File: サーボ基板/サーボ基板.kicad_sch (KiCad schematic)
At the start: 22 parts, among them J1 Conn_01x02, J2 Conn_01x03, J3 Conn_01x03, J4 Conn_01x03, J5 Conn_01x03, J6 DATA_IN, U1 SeeeduinoXIAO RP2040

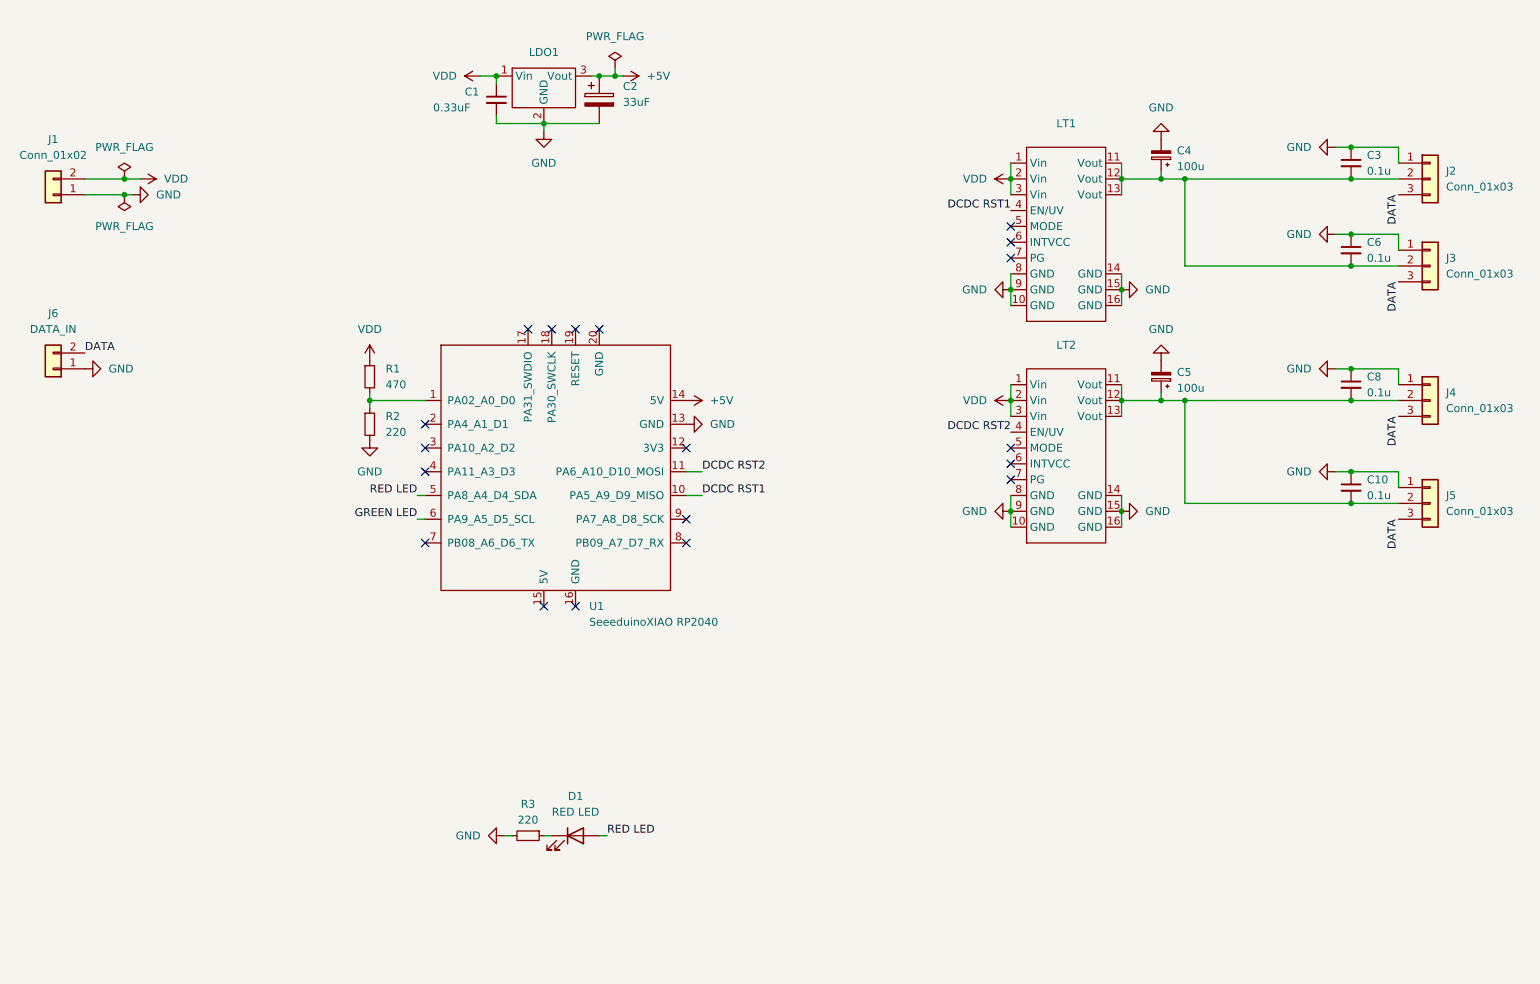
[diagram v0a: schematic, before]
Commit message: サーボ基板
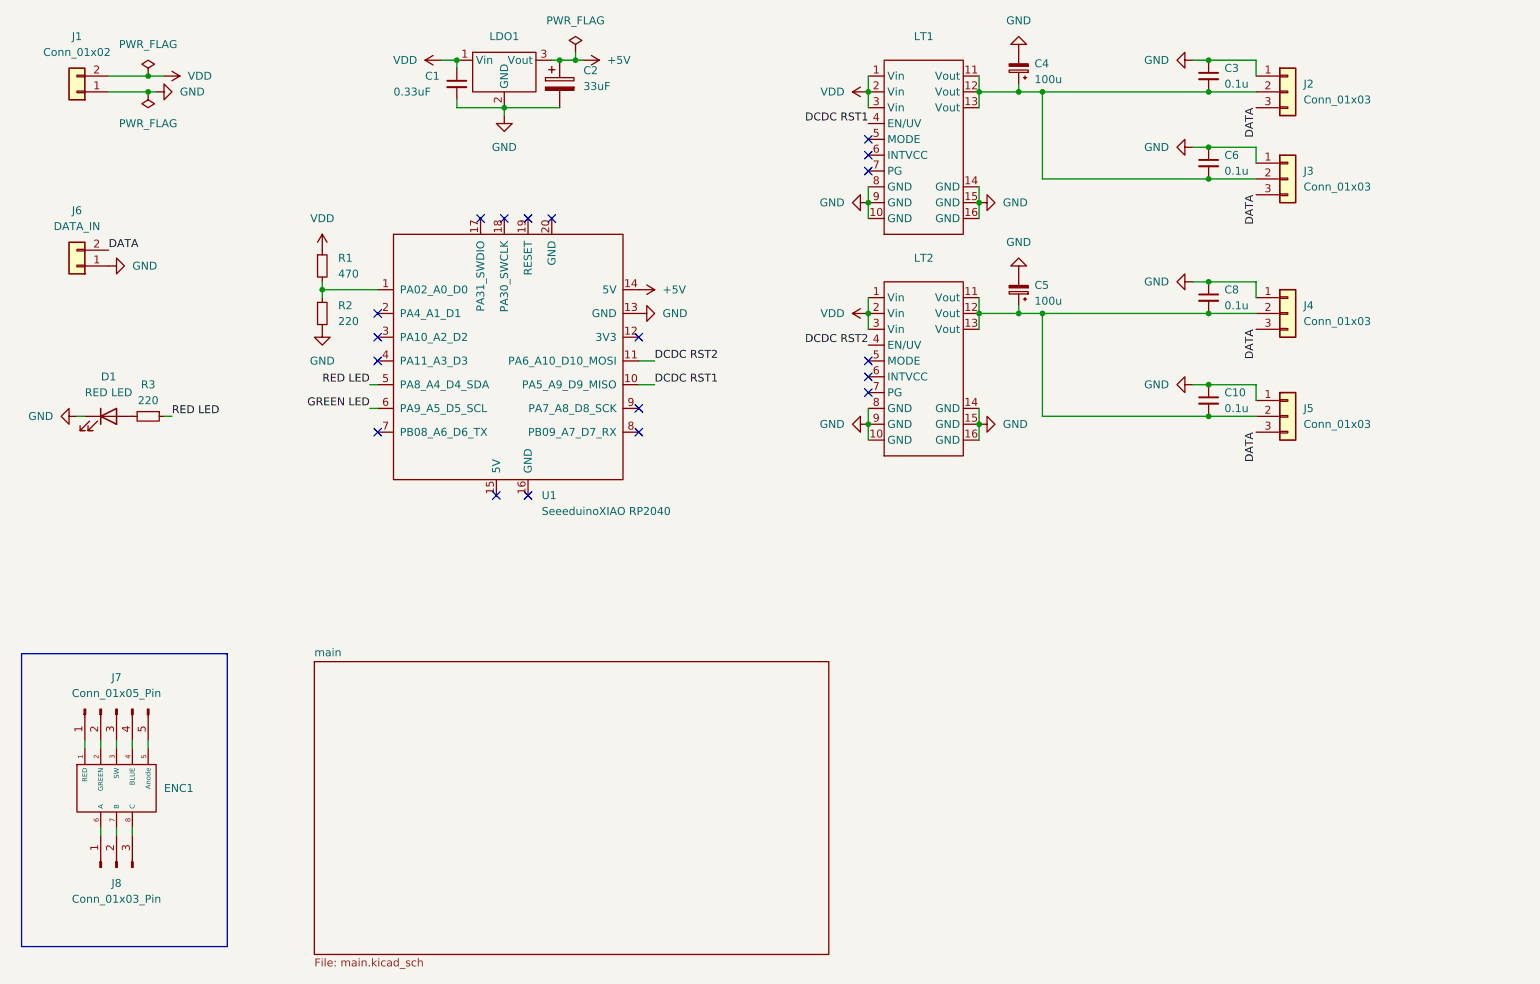
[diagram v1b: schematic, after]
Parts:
- added ENC1: ~, Potentiometer_LED:EC12PLRGBSDVBF, symbol Potentiometer_LED:EC12PLRGBSDVBF
- added J7: Conn_01x05_Pin, Connector_PinHeader_2.54mm:PinHeader_1x05_P2.54mm_Vertical, symbol Connector:Conn_01x05_Pin
- added J8: Conn_01x03_Pin, Connector_PinHeader_2.54mm:PinHeader_1x03_P2.54mm_Vertical, symbol Connector:Conn_01x03_Pin
- D1: footprint LED_THT:LED_D5.0mm_Horizontal_O1.27mm_Z3.0mm -> LED_THT:LED_D5.0mm
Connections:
- net GND: now also D1.1 (K); no longer R3.2
- net RED LED: now also R3.1; no longer D1.2 (A)
- new net: ENC1.6 (A), J8.1 (Pin_1)
- new net: ENC1.7 (B), J8.2 (Pin_2)
- new net: ENC1.8 (C), J8.3 (Pin_3)
- new net: ENC1.1 (RED), J7.1 (Pin_1)
- new net: ENC1.2 (GREEN), J7.2 (Pin_2)
- new net: ENC1.3 (SW), J7.3 (Pin_3)
- new net: ENC1.4 (BLUE), J7.4 (Pin_4)
- new net: ENC1.5 (Anode), J7.5 (Pin_5)
- new net: D1.2 (A), R3.2
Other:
- added sheet main (main.kicad_sch)
- moved on the sheet: C1, C10, C2, C3, C4, C5, C6, C8, D1, J1, J2, J3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
